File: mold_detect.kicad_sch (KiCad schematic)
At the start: 46 parts, among them J1 USB_C_Receptacle_USB2.0_14P, J2 ISP, U1 TPL5010, U2 FT230XS, U3 ATmega328P-P, U4 SHT30-DIS, U5 W25Q128JVS, Y1 16MHz

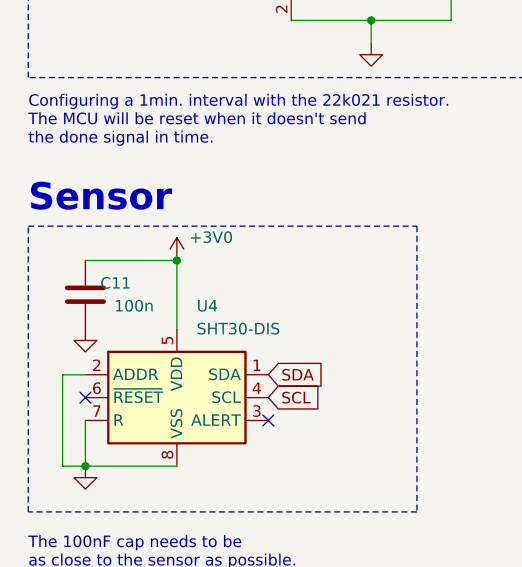
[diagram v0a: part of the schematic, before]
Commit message: added blender
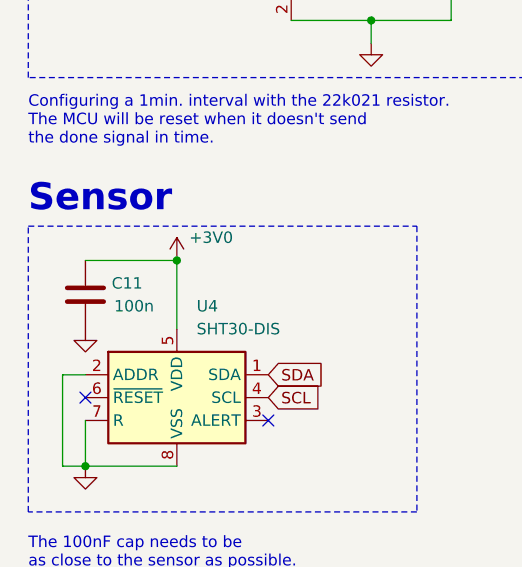
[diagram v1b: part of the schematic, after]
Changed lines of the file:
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@@
 		(at 278.13 173.99 0)
 		(unit 1)
-		(exclude_from_sim no)
+		(exclude_from_sim yes)
 		(in_bom no)
 		(on_board no)
@@
 		)
 		(property "Description" "Open Hardware logo, small"
-			(at 278.13 173.99 0)
-			(effects
-				(font
-					(size 1.27 1.27)
-				)
-				(hide yes)
-			)
-		)
-		(property "Sim.Enable" "0"
 			(at 278.13 173.99 0)
 			(effects
@@
 		(dnp no)
 		(property "Reference" "C11"
-			(at 25.4 76.2 0)
-			(effects
-				(font
+			(at 26.67 76.2 0)
+			(effects
+				(font
